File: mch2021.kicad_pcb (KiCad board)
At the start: 2 copper layers, 113.6 x 145.9 mm, 132 parts, among them J1 USB_OTG, J2 AudioJack3, J3 QG-2864KLBEG01, J4 Conn_02x03_Odd_Even, J5 Conn_02x05_Odd_Even, J6 Micro_SD_Card, Q1 Q_DUAL_NPN_NPN_E1B1C2E2B2C1, SW1 SW_SPDT, SW2 RESET_SW, SW3 BL_SWITCH, SW4 SW_SPDT, U1 XT4054K421MR-G, U10 MPR121Q, U11 SY6280AAC, U2 CH340C, U3 SY6280AAC, U4 SY8079, U5 PCM5100, U6 ESP32-WROVER, U7 74LVC1G17, U8 IR1261

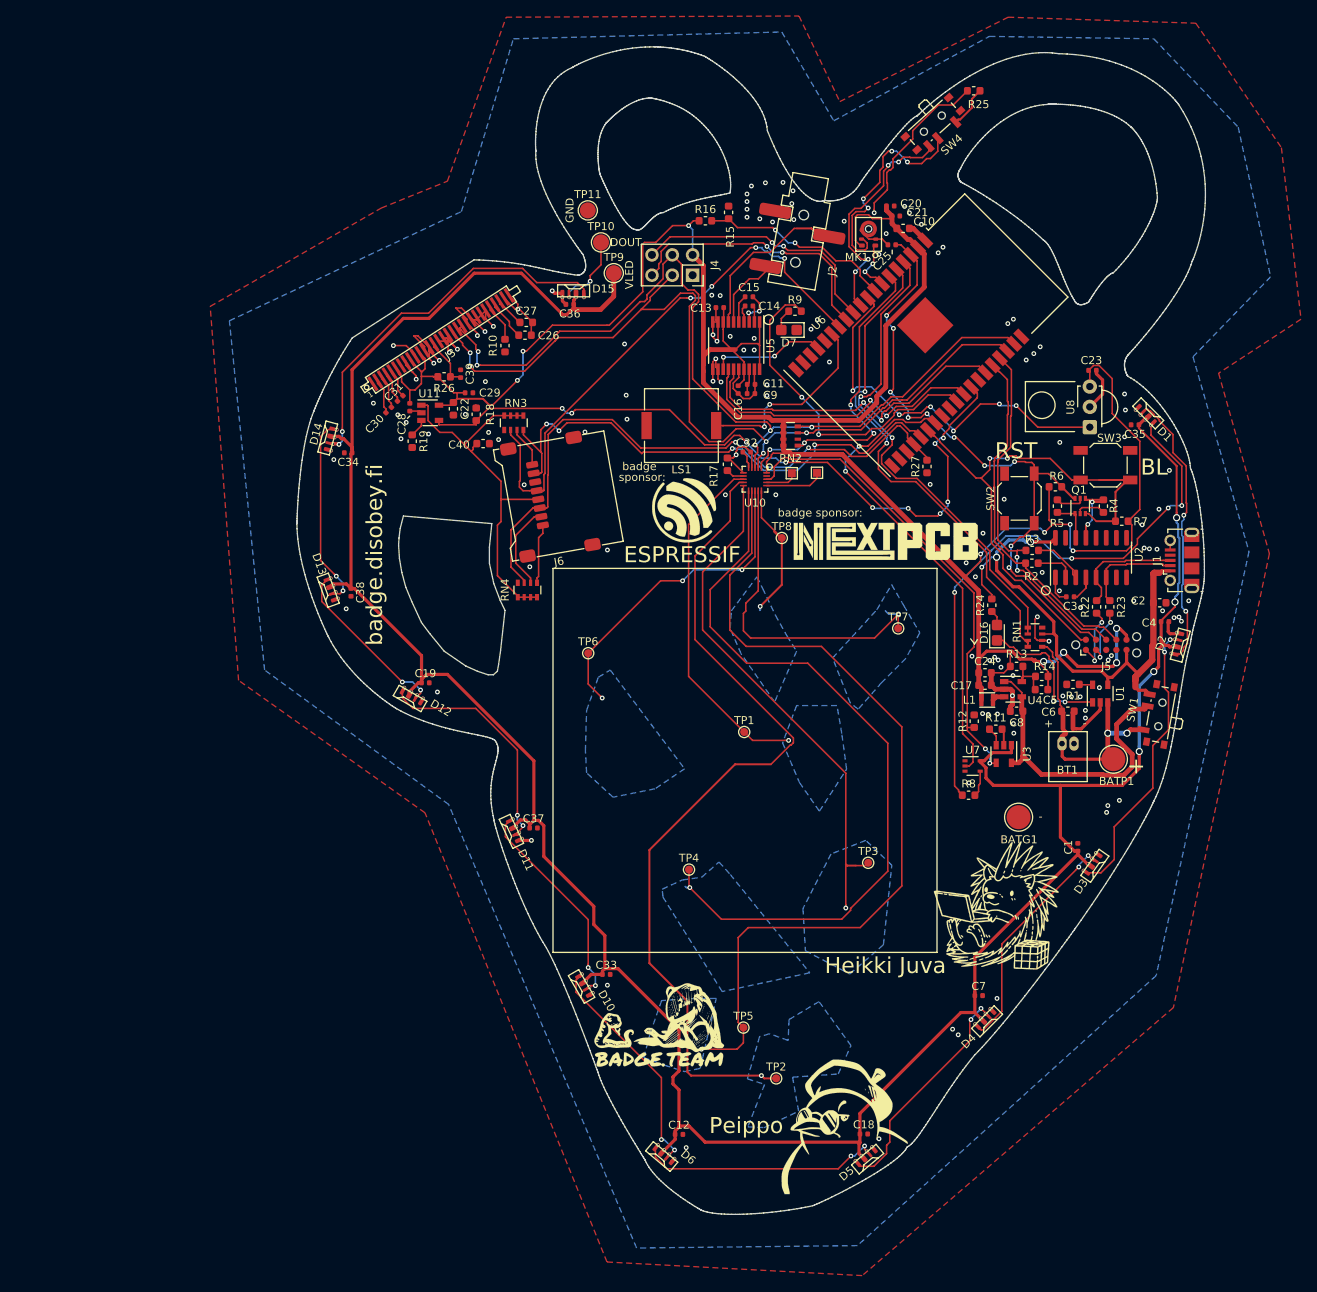
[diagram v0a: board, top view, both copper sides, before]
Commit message: Dump.
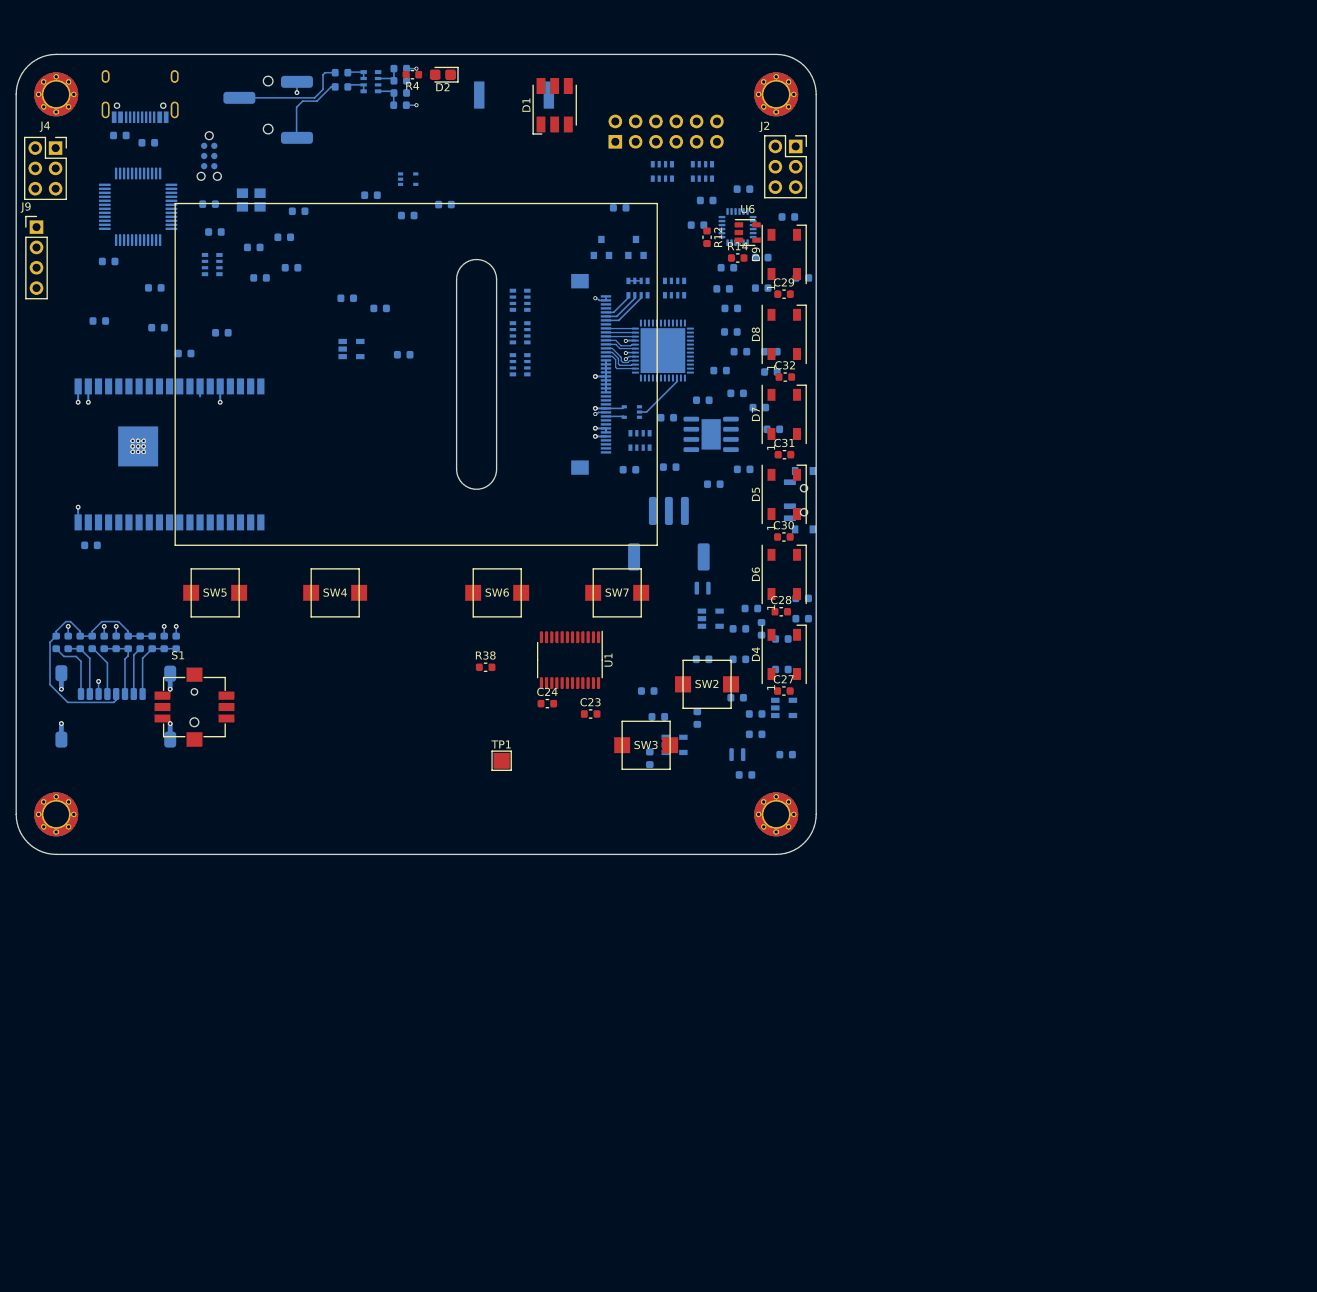
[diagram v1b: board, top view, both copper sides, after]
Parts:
- removed BATG1, BATP1: TestPoint_Flag, TestPoint:TestPoint_Pad_D3.0mm
- removed C22: 100p, Capacitor_SMD:C_0603_1608Metric
- removed C3: 100n, Capacitor_SMD:C_0402_1005Metric
- removed D10, D11, D12, D13, D14, D15: WS2812B, corelib:SK6212SIDE
- removed D16: LED, LED_SMD:LED_0805_2012Metric_Castellated
- removed G***: LOGO, disobey-logo
- removed G***: LOGO, peippo
- removed G***: LOGO, nextpcb
- removed G***: LOGO, badgeteam
- removed G***: LOGO, heikki
- removed G***: LOGO, espressif
- removed G***: LOGO, corp-silk
- removed G***: LOGO, corp-mask
- removed MK1: SPH0641LM4H-1, corelib:Knowles-SPH0641LM4H-1
- removed REF** (x2): TestPoint_Pad_1.0x1.0mm, TestPoint:TestPoint_Pad_1.0x1.0mm
- removed REF**: Battery-48x48mm, corelib:Battery-48x48mm
- removed RN3, RN4: 10k, Resistor_SMD:R_Array_Convex_4x0603
- removed TP10, TP11, TP9: TestPoint, TestPoint:TestPoint_Pad_D2.0mm
- removed TP2, TP3, TP4, TP5, TP6, TP7, TP8: TestPoint_Flag, TestPoint:TestPoint_Pad_D1.0mm
- removed U8: IR1261, OptoDevice:Vishay_MINICAST-3Pin
- added C41: 100n, Capacitor_SMD:C_0603_1608Metric, B.Cu at (90.1, 42.4)
- added C42: 100n, Capacitor_SMD:C_0603_1608Metric, B.Cu at (81.7, 51.6)
- added C43: 20p, Capacitor_SMD:C_0603_1608Metric, B.Cu at (29.7, 24.1)
- added C44: 20p, Capacitor_SMD:C_0603_1608Metric, B.Cu at (33.5, 22.9)
- added C45: 100n, Capacitor_SMD:C_0603_1608Metric, B.Cu at (34.4, 26.7)
- added C46: 100n, Capacitor_SMD:C_0603_1608Metric, B.Cu at (11.6, 25.9)
- added C47: 100n, Capacitor_SMD:C_0603_1608Metric, B.Cu at (30.5, 27.9)
- added D8: WS2812B, LED_SMD:LED_WS2812B_PLCC4_5.0x5.0mm_P3.2mm, F.Cu at (96.0, 35.0)
- added D9: WS2812B, LED_SMD:LED_WS2812B_PLCC4_5.0x5.0mm_P3.2mm, F.Cu at (96.0, 25.0)
- added H1: MountingHole_Pad, corecode:HOLE-M3-COND, F.Cu at (5.00, 5.00)
- added H2: MountingHole_Pad, corecode:HOLE-M3-COND, F.Cu at (95.0, 5.00)
- added H3: MountingHole_Pad, corecode:HOLE-M3-COND, F.Cu at (5.00, 95.0)
- added H4: MountingHole_Pad, corecode:HOLE-M3-COND, F.Cu at (95.0, 95.0)
- added J7: LCD, Connector_FFC-FPC:Hirose_FH12-40S-0.5SH_1x40-1MP_P0.50mm_Horizontal, B.Cu at (71.9, 40.0)
- added J8: PROG, Connector:Tag-Connect_TC2030-IDC-NL_2x03_P1.27mm_Vertical, B.Cu at (24.1, 12.7)
- added J9: GPIO, Connector_PinHeader_2.54mm:PinHeader_1x04_P2.54mm_Vertical, F.Cu at (2.54, 21.6)
- added L2: 2.2u, custom:Inductor_MSC20FC, B.Cu at (90.1, 87.5)
- added Q2: Q_NMOS_GSD, Package_TO_SOT_SMD:SOT-23, B.Cu at (73.2, 24.1)
- added R20: DNP, Resistor_SMD:R_0603_1608Metric, B.Cu at (20.0, 73.5)
- added R21: DNP, Resistor_SMD:R_0603_1608Metric, B.Cu at (12.5, 73.5)
- added R28: 100k, Resistor_SMD:R_0603_1608Metric, B.Cu at (88.0, 39.5)
- added R29: TBD, Resistor_SMD:R_0603_1608Metric, B.Cu at (48.0, 4.83)
- added R30: TBD, Resistor_SMD:R_0603_1608Metric, B.Cu at (48.0, 3.30)
- added R31: 10k, Resistor_SMD:R_0603_1608Metric, B.Cu at (90.5, 37.2)
- added R32: 10k, Resistor_SMD:R_0603_1608Metric, B.Cu at (44.3, 17.6)
- added R33: 10k, Resistor_SMD:R_0603_1608Metric, B.Cu at (48.9, 20.1)
- added R34: 10k, Resistor_SMD:R_0603_1608Metric, B.Cu at (35.3, 19.6)
- added R35: 10k, Resistor_SMD:R_0603_1608Metric, B.Cu at (24.1, 18.7)
- added R36: 10k, Resistor_SMD:R_0603_1608Metric, B.Cu at (17.3, 29.2)
- added R37: 4k7, Resistor_SMD:R_0603_1608Metric, B.Cu at (85.8, 43.2)
- added R38: 4k7, Resistor_SMD:R_0603_1608Metric, F.Cu at (58.7, 76.6)
- added R49: 10k, Resistor_SMD:R_0603_1608Metric, B.Cu at (10.4, 33.3)
- added R50: 10k, Resistor_SMD:R_0603_1608Metric, B.Cu at (25.7, 34.8)
- added R51: 10k, Resistor_SMD:R_0603_1608Metric, B.Cu at (48.4, 37.5)
- added R52: 10k, Resistor_SMD:R_0603_1608Metric, B.Cu at (21.1, 37.4)
- added R53: 10k, Resistor_SMD:R_0603_1608Metric, B.Cu at (9.50, 73.5)
- added R54: 10k, Resistor_SMD:R_0603_1608Metric, B.Cu at (14.0, 73.5)
- added R55: 10k, Resistor_SMD:R_0603_1608Metric, B.Cu at (8.00, 73.5)
- added R56: 10k, Resistor_SMD:R_0603_1608Metric, B.Cu at (5.00, 73.5)
- added R57: 10k, Resistor_SMD:R_0603_1608Metric, B.Cu at (17.0, 73.5)
- added R58: 10k, Resistor_SMD:R_0603_1608Metric, B.Cu at (15.5, 73.5)
- added RN10: 100k, Resistor_SMD:R_Array_Convex_4x0603, B.Cu at (63.0, 30.7)
- added RN11: 100k, Resistor_SMD:R_Array_Convex_4x0603, B.Cu at (63.0, 38.8)
- added RN12: 100k, Resistor_SMD:R_Array_Convex_4x0603, B.Cu at (63.0, 34.8)
- added RN13: 47, Resistor_SMD:R_Array_Convex_4x0603, B.Cu at (85.8, 14.6)
- added RN14: 47, Resistor_SMD:R_Array_Convex_4x0603, B.Cu at (80.8, 14.6)
- added RN7: 47, Resistor_SMD:R_Array_Convex_4x0603, B.Cu at (78.0, 48.3)
- added RN8: 47, Resistor_SMD:R_Array_Convex_4x0603, B.Cu at (77.7, 29.2)
- added RN9: 100k, Resistor_SMD:R_Array_Convex_4x0603, B.Cu at (82.3, 29.2)
- added S1: JS1400BFQ, custom:SW_JS1400BFQ, F.Cu at (22.3, 81.6)
- added SW5: Home, custom:1TS009, F.Cu at (24.9, 67.3)
- added SW6: Start, custom:1TS009, F.Cu at (60.1, 67.3)
- added SW7: Select, custom:1TS009, F.Cu at (75.1, 67.3)
- added U12: LY68L6400, Package_SO:SOIC-8-1EP_3.9x4.9mm_P1.27mm_EP2.41x3.81mm, B.Cu at (86.9, 47.5)
- added U13: 74LVC1G125, Package_TO_SOT_SMD:SOT-353_SC-70-5, B.Cu at (49.0, 15.6)
- added U14: STM32F103C8Tx, Package_QFP:LQFP-48_7x7mm_P0.5mm, B.Cu at (15.2, 19.1)
- added U9: ESP32-WROVER, custom:ESP32-WROVER, B.Cu at (16.0, 50.0)
- added Y1: 16MHz, Crystal:Crystal_SMD_3225-4Pin_3.2x2.5mm, B.Cu at (29.4, 18.2)
- BT1: value Battery_Cell -> LiPo; footprint corelib:S2B-ZR -> Connector_JST:JST_PH_S3B-PH-SM4-TB_1x03-1MP_P2.00mm_Horizontal; moved to B.Cu
- C1, C36, C37: value 1u -> C_Small; footprint Capacitor_SMD:C_0402_1005Metric -> Capacitor_SMD:C_0603_1608Metric; moved to B.Cu
- C10, C6: value 10u -> 22u; moved to B.Cu
- C11, C13: value 100n -> 22u; footprint Capacitor_SMD:C_0402_1005Metric -> Capacitor_SMD:C_0603_1608Metric; moved to B.Cu
- C12, C16: value 1u -> 22u; footprint Capacitor_SMD:C_0402_1005Metric -> Capacitor_SMD:C_0603_1608Metric; moved to B.Cu
- C14, C21, C34, C4: value 1u -> 10u; footprint Capacitor_SMD:C_0402_1005Metric -> Capacitor_SMD:C_0603_1608Metric; moved to B.Cu
- C15, C18, C33, C35, C38, C39, C7: value 1u -> 100n; footprint Capacitor_SMD:C_0402_1005Metric -> Capacitor_SMD:C_0603_1608Metric; moved to B.Cu
- C17, C40: value 22u -> 100n; moved to B.Cu
- C19: value 1u -> 2.2n; footprint Capacitor_SMD:C_0402_1005Metric -> Capacitor_SMD:C_0603_1608Metric; moved to B.Cu
- C2: value 10u -> C_Small; moved to B.Cu
- C20, C25: footprint Capacitor_SMD:C_0402_1005Metric -> Capacitor_SMD:C_0603_1608Metric; moved to B.Cu
- C23: value 1u -> 100n; footprint Capacitor_SMD:C_0402_1005Metric -> Capacitor_SMD:C_0603_1608Metric
- C24: value 22u -> 10u
- C26: value 4.7u -> 10u; moved to B.Cu
- C27: value 2.2u -> 1u
- C28, C29, C30, C31: footprint Capacitor_SMD:C_0402_1005Metric -> Capacitor_SMD:C_0603_1608Metric
- C32: value 100n -> 1u; footprint Capacitor_SMD:C_0402_1005Metric -> Capacitor_SMD:C_0603_1608Metric
- C5: value 22p -> 22u; moved to B.Cu
- C8: value 22u -> 22p; moved to B.Cu
- C9: value 1u -> 22p; footprint Capacitor_SMD:C_0402_1005Metric -> Capacitor_SMD:C_0603_1608Metric; moved to B.Cu
- D1: value WS2812B -> RGB-5050; footprint corelib:SK6212SIDE -> LED_SMD:LED_RGB_5050-6
- D2: value WS2812B -> LED; footprint corelib:SK6212SIDE -> LED_SMD:LED_0805_2012Metric_Castellated
- D3: value WS2812B -> CDBU0130R; footprint corelib:SK6212SIDE -> Diode_SMD:D_0603_1608Metric; moved to B.Cu
- D4, D5, D6: footprint corelib:SK6212SIDE -> LED_SMD:LED_WS2812B_PLCC4_5.0x5.0mm_P3.2mm
- D7: value LED -> WS2812B; footprint LED_SMD:LED_0805_2012Metric_Castellated -> LED_SMD:LED_WS2812B_PLCC4_5.0x5.0mm_P3.2mm
- J1: value USB_OTG -> USB_C_Receptacle_USB2.0; footprint Connector_USB:USB_Micro-B_Molex-105017-0001 -> Connector_USB:USB_C_Receptacle_HRO_TYPE-C-31-M-12; moved to B.Cu
- J2: value AudioJack3 -> SAO; footprint corelib:Boom-audiojack-PJ-320B -> Connector_PinSocket_2.54mm:PinSocket_2x03_P2.54mm_Vertical
- J3: value QG-2864KLBEG01 -> AudioJack3; footprint corelib:hotbar_30x0.7 -> custom:Boom-audiojack-PJ-320B; moved to B.Cu
- J4: value Conn_02x03_Odd_Even -> SAO
- J5: value Conn_02x05_Odd_Even -> Micro SD card; footprint Connector:Tag-Connect_TC2050-IDC-NL_2x05_P1.27mm_Vertical -> custom:MicroSD-SOFNG-TF-002-H18; moved to B.Cu
- J6: value Micro_SD_Card -> PMOD; footprint corelib:MicroSD-SOFNG-TF-002-H18 -> Connector_PinSocket_2.54mm:PinSocket_2x06_P2.54mm_Horizontal; moved to B.Cu
- L1: footprint corelib:Inductor_MSC20FC -> custom:Inductor_MSC20FC; moved to B.Cu
- LS1, R13, R6, R7: moved to B.Cu
- Q1: value Q_DUAL_NPN_NPN_E1B1C2E2B2C1 -> Q_NMOS_GSD; footprint Package_TO_SOT_SMD:SOT-363_SC-70-6 -> Package_TO_SOT_SMD:SOT-23; moved to B.Cu
- R1: value 2k -> 5k1; moved to B.Cu
- R10: value 910k -> 2k; moved to B.Cu
- R11: value 3.4k -> 10k; moved to B.Cu
- R14: value 45.3k -> 3.4k
- R15: value R -> 4k7; moved to B.Cu
- R16: value 10k -> 4k7; moved to B.Cu
- R17: value 75k -> 4k7; moved to B.Cu
- R18, R19: value 10k -> 45.3k; moved to B.Cu
- R2: value 100R -> 5k1; moved to B.Cu
- R22: value 0 -> 45.3k; moved to B.Cu
- R23: value 0 -> 47; moved to B.Cu
- R24: value 2K -> 47; moved to B.Cu
- R25: value 10k -> 100k; moved to B.Cu
- R26: value 10k -> 100; moved to B.Cu
- R27: value 45.3k -> 100k; moved to B.Cu
- R3: value 100R -> 47; moved to B.Cu
- R4: value 10k -> 100
- R5: value 10k -> 2k; moved to B.Cu
- R8: value 1k -> 45.3k; moved to B.Cu
- R9: value 100R -> 10k; moved to B.Cu
- RN1: value 100k -> TBD; moved to B.Cu
- RN2: value 4.7k -> 100k; moved to B.Cu
- SW1: value SW_SPDT -> Power switch; moved to B.Cu
- SW2: value RESET_SW -> Accept; footprint Button_Switch_SMD:SW_SPST_SKQG_WithStem -> custom:1TS009
- SW3: value BL_SWITCH -> Back; footprint Button_Switch_SMD:SW_SPST_SKQG_WithStem -> custom:1TS009
- SW4: value SW_SPDT -> Menu; footprint Button_Switch_SMD:SW_SPDT_PCM12 -> custom:1TS009
- TP1: value TestPoint_Flag -> IOEXP; footprint TestPoint:TestPoint_Pad_D1.0mm -> TestPoint:TestPoint_Pad_2.0x2.0mm
- U1: value XT4054K421MR-G -> PCA9555PW; footprint Package_TO_SOT_SMD:SOT-23-5 -> Package_SO:TSSOP-24_4.4x7.8mm_P0.65mm
- U10: value MPR121Q -> 74LVC1G125; footprint Package_DFN_QFN:QFN-20-1EP_3x3mm_P0.4mm_EP1.65x1.65mm -> Package_TO_SOT_SMD:SOT-353_SC-70-5; moved to B.Cu
- U11: value SY6280AAC -> ICE40UP5K-SG48ITR; footprint Package_TO_SOT_SMD:SOT-23-5 -> Package_DFN_QFN:QFN-48-1EP_7x7mm_P0.5mm_EP5.6x5.6mm; moved to B.Cu
- U2: value CH340C -> SY8079AAC; footprint Package_SO:SOIC-16_3.9x9.9mm_P1.27mm -> Package_TO_SOT_SMD:SOT-23-5; moved to B.Cu
- U3: value SY6280AAC -> SY8079AAC; moved to B.Cu
- U4: value SY8079 -> XT4054K421MR-G; moved to B.Cu
- U5: value PCM5100 -> SY6280AAC; footprint Package_SO:TSSOP-20_4.4x6.5mm_P0.65mm -> Package_TO_SOT_SMD:SOT-23-5; moved to B.Cu
- U6: value ESP32-WROVER -> SY6280AAC; footprint corelib:ESP32-WROVER -> Package_TO_SOT_SMD:SOT-23-5
- U7: value 74LVC1G17 -> MPU-6050; footprint Package_TO_SOT_SMD:SOT-353_SC-70-5 -> Sensor_Motion:InvenSense_QFN-24_4x4mm_P0.5mm; moved to B.Cu
- moved J1 143.1 mm to (15.5, 3.81), turned to 0 degrees
- moved R1 137.5 mm to (13.0, 10.1), turned to 0 degrees
- moved C1 132.3 mm to (40.7, 4.06), turned to 180 degrees
- moved R22 124.1 mm to (11.0, 73.5)
- moved J5 123.9 mm to (12.5, 80.0)
- moved R2 122.3 mm to (16.5, 11.0)
- moved C2 121.9 mm to (40.7, 2.29)
- moved D2 117.0 mm to (53.3, 2.54), turned to 180 degrees
- moved C18 110.3 mm to (93.2, 25.4)
- moved RN1 108.2 mm to (44.3, 3.41), turned to 0 degrees
- moved D3 101.8 mm to (75.4, 19.2), turned to 0 degrees
- moved R4 101.8 mm to (49.5, 2.54), turned to 180 degrees
- moved R11 97.3 mm to (41.4, 30.5)
- moved C37 96.4 mm to (48.0, 1.78), turned to 180 degrees
- moved SW4 95.0 mm to (39.9, 67.3), turned to 0 degrees
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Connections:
- BT1 pad 1: /BAT -> +3V3
- C1 pad 1: VCC -> Net-(C1-Pad1)
- C1 pad 2: GND -> Net-(C1-Pad2)
- C10 pad 1: /3V3 -> +3V3
- C11 pad 1: Net-(C11-Pad1) -> +1V2
- C12 pad 1: VCC -> +3V3
- C13 pad 1: /3V3 -> +1V2
- C14 pad 1: Net-(C14-Pad1) -> +3V3
- C14 pad 2: Net-(C14-Pad2) -> GND
- C15 pad 1: Net-(C15-Pad1) -> +3V3
- C16 pad 1: /3V3 -> PWR_SDCARD
- C17 pad 1: /3V3 -> +3V3
- C18 pad 1: VCC -> GND
- C18 pad 2: GND -> Net-(C18-Pad2)
- C19 pad 1: VCC -> GND
- C19 pad 2: GND -> Net-(C19-Pad2)
- C2 pad 1: /VUSB -> Net-(C2-Pad1)
- C2 pad 2: GND -> Net-(C2-Pad2)
- C20 pad 1: /3V3 -> +3V3
- C21 pad 1: /3V3 -> +3V3
- C23 pad 1: GND -> +3V3
- C23 pad 2: /3V3 -> GND
- C24 pad 1: /3V3 -> +3V3
- C25 pad 1: /RESET -> +3V3
- C26 pad 1: Net-(C26-Pad1) -> +3V3
- C27 pad 1: Net-(C27-Pad1) -> PWR_LED
- C28 pad 1: /3V3 -> PWR_LED
- C29 pad 1: /3V3 -> PWR_LED
- C30 pad 1: Net-(C30-Pad1) -> PWR_LED
- C30 pad 2: Net-(C30-Pad2) -> GND
- C31 pad 1: Net-(C31-Pad1) -> PWR_LED
- C31 pad 2: Net-(C31-Pad2) -> GND
- C32 pad 1: Net-(C32-Pad1) -> PWR_LED
- C33 pad 1: VCC -> +1V2
- C34 pad 1: VCC -> Net-(C34-Pad1)
- C35 pad 1: VCC -> Net-(C34-Pad1)
- C36 pad 1: VCC -> GND
- C36 pad 2: GND -> /FPGA/AUDO_L
- C37 pad 1: VCC -> GND
- C37 pad 2: GND -> /FPGA/AUDO_R
- C38 pad 1: VCC -> +3V3
- C39 pad 1: GND -> +3V3
- C39 pad 2: Net-(C39-Pad2) -> GND
- C4 pad 1: VCC -> GND
- C4 pad 2: GND -> VUSB
- C40 pad 1: /GATEDPOWER -> +3V3
- C5 pad 1: /3V3 -> VIN
- C5 pad 2: Net-(C5-Pad2) -> GND
- C6 pad 1: /BAT -> VIN
- C7 pad 1: VCC -> GND
- C7 pad 2: GND -> VUSB
- C8 pad 1: /BATSW -> +3V3
- C8 pad 2: GND -> /POWER/FB33
- C9 pad 1: Net-(C11-Pad1) -> +1V2
- C9 pad 2: GND -> /POWER/FB12
- D1 pad 1: VCC -> /FPGA/RGB2
- D1 pad 2: Net-(D1-Pad2) -> /FPGA/RGB0
- D1 pad 3: GND -> /FPGA/RGB1
- D1 pad 4: /LED_DIN -> +3V3
- D2 pad 1: VCC -> GND
- D3 pad 1: VCC -> +2V5
- D3 pad 2: Net-(D3-Pad2) -> +3V3
- D4 pad 1: VCC -> PWR_LED
- D4 pad 4: Net-(D3-Pad2) -> /LED/DATA_IN
- D5 pad 1: VCC -> PWR_LED
- D6 pad 1: VCC -> PWR_LED
- D6 pad 2: Net-(D10-Pad4) -> Net-(D6-Pad2)
- D7 pad 1: GND -> PWR_LED
- J4 pad 2: /3V3 -> +3V3
- J4 pad 3: /SCL -> /ACCELEROMETER/I2C_SCL
- J4 pad 4: /SDA -> /ACCELEROMETER/I2C_SDA
- J4 pad 5: Net-(J4-Pad5) -> /STM32/SAO_IO0
- J4 pad 6: Net-(J4-Pad6) -> /STM32/SAO_IO1
- J5 pad 1: Net-(J5-Pad1) -> SD_D2
- J5 pad 2: Net-(J5-Pad2) -> /ESP32/SD_D3
- J5 pad 3: GND -> SD_CMD
- J5 pad 4: GND -> PWR_SDCARD
- J5 pad 5: /VUSB -> /ESP32/SD_CLK
- J5 pad 6: /3V3 -> GND
- J5 pad 7: /ESPRX -> SD_D0
- J5 pad 8: /ESPTX -> /ESP32/SD_D1
- J5 pad 9: /RESET -> GND
- J6 pad 1: Net-(J6-Pad1) -> +3V3
- J6 pad 2: Net-(J6-Pad2) -> +3V3
- J6 pad 3: /SD_CMD -> GND
- J6 pad 4: /GATEDPOWER -> GND
- J6 pad 5: /SD_CLK -> /FPGA/PMOD_8
- J6 pad 6: GND -> /FPGA/PMOD_4
- J6 pad 7: /SD_D0 -> /FPGA/PMOD_7
- J6 pad 8: Net-(J6-Pad8) -> /FPGA/PMOD_3
- J6 pad 9: GND -> /FPGA/PMOD_6
- L1 pad 1: /3V3 -> +3V3
- L1 pad 2: Net-(L1-Pad2) -> /POWER/SW33
- LS1 pad 1: /BUZZER -> GND
- LS1 pad 2: GND -> SPK
- Q1 pad 2: Net-(Q1-Pad2) -> GND
- Q1 pad 3: /BL -> Net-(Q1-Pad3)
- R1 pad 1: Net-(R1-Pad1) -> GND
- R1 pad 2: GND -> /CC1
- R10 pad 1: Net-(J3-Pad26) -> /POWER/CHARGING
- R10 pad 2: GND -> +3V3
- R11 pad 1: Net-(R11-Pad1) -> GND
- R11 pad 2: GND -> /ESP32/PWR_SDCARD_ENABLE
- R12 pad 1: /LEDON -> GND
- R12 pad 2: GND -> /POWER/PWR_LED_ENABLE
- R13 pad 1: Net-(C5-Pad2) -> GND
- R13 pad 2: GND -> Net-(R13-Pad2)
- R14 pad 1: /3V3 -> Net-(R14-Pad1)
- R14 pad 2: Net-(C5-Pad2) -> GND
- R15 pad 1: Net-(R15-Pad1) -> +3V3
- R15 pad 2: GND -> /ACCELEROMETER/AUX_SDA
- R16 pad 1: /3V3 -> +3V3
- R16 pad 2: Net-(R15-Pad1) -> /ACCELEROMETER/AUX_SCL
- R17 pad 1: Net-(R17-Pad1) -> +3V3
- R17 pad 2: GND -> /ACCELEROMETER/IRQ
- R18 pad 1: Net-(R18-Pad1) -> SD_D0
- R19 pad 1: Net-(R19-Pad1) -> +3V3
- R19 pad 2: GND -> SD_D2
- R2 pad 1: /ESPRX -> GND
- R2 pad 2: Net-(R2-Pad2) -> /CC2
- R22 pad 1: Net-(J5-Pad1) -> SD_CMD
- R22 pad 2: /D_P -> GND
- R23 pad 1: /D_N -> /LCD/LCD_RS_SCK
- R23 pad 2: Net-(J5-Pad2) -> /FPGA/LCD_RS
- R24 pad 1: Net-(D16-Pad2) -> /LCD/LCD_IM0
- R24 pad 2: /VUSB -> /STM32/LCD_MODE
- R25 pad 1: GND -> /FPGA/SPI_CS
- R25 pad 2: Net-(R25-Pad2) -> GND
- R26 pad 1: Net-(C39-Pad2) -> +1V2
- R26 pad 2: /3V3 -> Net-(C34-Pad1)
- R27 pad 1: GND -> /BUTTONS/FPGA_RESET
- R27 pad 2: /SD_CMD -> GND
- R3 pad 1: /ESPTX -> Net-(J2-Pad6)
- R3 pad 2: Net-(R3-Pad2) -> /LED/DATA_OUT
- R4 pad 1: Net-(Q1-Pad2) -> Net-(D2-Pad2)
- R4 pad 2: Net-(Q1-Pad4) -> /ESP32/IR_TX
- R5 pad 1: Net-(Q1-Pad5) -> Net-(R5-Pad1)
- R5 pad 2: Net-(Q1-Pad1) -> GND
- R6 pad 1: /RESET -> /POWER/FB33
- R6 pad 2: /3V3 -> GND
- R7 pad 1: /BL -> /POWER/FB12
- R7 pad 2: /3V3 -> GND
- R8 pad 1: /LED_DIN -> +3V3
- R8 pad 2: Net-(R8-Pad2) -> /POWER/FB33
- R9 pad 1: Net-(D7-Pad2) -> +1V2
- R9 pad 2: /IR_SEND -> /POWER/FB12
- RN1 pad 1: /BAT -> Net-(C1-Pad1)
- RN1 pad 2: GND -> Net-(C1-Pad1)
- RN1 pad 3: /VUSB -> Net-(C2-Pad2)
- RN1 pad 4: GND -> Net-(C2-Pad2)
- RN1 pad 5: /USB_SENSE -> ESP32_AUDIO_R
- RN1 pad 6: /USB_SENSE -> /FPGA/AUDO_R
- RN1 pad 7: /BATSENSE -> ESP32_AUDIO_L
- RN1 pad 8: /BATSENSE -> /FPGA/AUDO_L
- RN2 pad 1: /TOUCHRDY -> +3V3
- RN2 pad 2: Net-(RN2-Pad2) -> GND
- RN2 pad 3: /SCL -> VUSB
- RN2 pad 4: /SDA -> GND
- RN2 pad 5: /3V3 -> /POWER/SENSE_VUSB
- RN2 pad 6: /3V3 -> /POWER/SENSE_VUSB
- RN2 pad 7: /3V3 -> /POWER/SENSE_VBAT
- RN2 pad 8: /3V3 -> /POWER/SENSE_VBAT
- SW1 pad 1: /BAT -> +3V3
- SW1 pad 2: /BATSW -> VIN
- SW1 pad 3: /VUSB -> VUSB
- SW2 pad 1: GND -> Net-(SW2-Pad1)
- SW2 pad 2: /RESET -> GND
- SW3 pad 1: GND -> Net-(SW3-Pad1)
- SW3 pad 2: /BL -> GND
- SW4 pad 1: Net-(R25-Pad2) -> Net-(SW4-Pad1)
- SW4 pad 2: Net-(MK1-Pad4) -> GND
- TP1 pad 1: /T-UP -> Net-(TP1-Pad1)
- U1 pad 1: Net-(D16-Pad1) -> /BUTTONS/IRQ
- U1 pad 3: /BAT -> GND
- U1 pad 4: /VUSB -> Net-(S1-Pad1)
- U1 pad 5: Net-(R1-Pad1) -> Net-(S1-Pad2)
- U10 pad 1: /TOUCHRDY -> /LCD/LCD_RS_SCK_SWITCH
- U10 pad 2: /SCL -> /ESP32/SPI_CLK
- U10 pad 3: /SDA -> GND
- U10 pad 4: GND -> /LCD/LCD_RS_SCK
- U10 pad 5: Net-(C32-Pad1) -> +3V3
- U11 pad 1: /GATEDPOWER -> +3V3
- U11 pad 2: GND -> Net-(RN14-Pad3)
- U11 pad 3: Net-(R19-Pad1) -> Net-(RN14-Pad1)
- U11 pad 4: Net-(R18-Pad1) -> Net-(RN14-Pad2)
- U11 pad 5: /3V3 -> +1V2
- U2 pad 1: GND -> VIN
- U2 pad 2: Net-(R2-Pad2) -> GND
- U2 pad 3: Net-(R3-Pad2) -> /POWER/SW33
- U2 pad 4: Net-(C3-Pad1) -> VIN
- U2 pad 5: /D_P -> /POWER/FB33
- U3 pad 1: VCC -> VIN
- U3 pad 3: Net-(R11-Pad1) -> /POWER/SW12
- U3 pad 4: /LEDON -> VIN
- U3 pad 5: /BATSW -> /POWER/FB12
- U4 pad 1: /BATSW -> /POWER/CHARGING
- U4 pad 3: Net-(L1-Pad2) -> +3V3
- U4 pad 4: /BATSW -> VUSB
- U4 pad 5: Net-(C5-Pad2) -> Net-(R5-Pad1)
- U5 pad 1: /3V3 -> PWR_SDCARD
- U5 pad 2: Net-(C14-Pad1) -> GND
- U5 pad 3: GND -> Net-(R13-Pad2)
- U5 pad 4: Net-(C14-Pad2) -> /ESP32/PWR_SDCARD_ENABLE
- U5 pad 5: Net-(C15-Pad1) -> +3V3
- U6 pad 1: GND -> PWR_LED
- U6 pad 2: /3V3 -> GND
- U6 pad 3: /RESET -> Net-(R14-Pad1)
- U6 pad 4: /USB_SENSE -> /POWER/PWR_LED_ENABLE
- U6 pad 5: /BATSENSE -> +3V3
- U7 pad 1: (no net) -> GND
- U7 pad 2: Net-(U6-Pad26) -> (no net)
- U7 pad 3: GND -> (no net)
- U7 pad 4: Net-(R8-Pad2) -> (no net)
- U7 pad 5: VCC -> (no net)
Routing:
- net VCC: track 351.3 -> 0.00 mm, vias 4 -> 0
- net /3V3: track 323.1 -> 0.00 mm, vias 11 -> 0
- net GND: track 158.6 -> 29.6 mm, vias 134 -> 25
- net /SCL: track 112.1 -> 0.00 mm, vias 5 -> 0
- net /SDA: track 111.7 -> 0.00 mm, vias 5 -> 0
- net /T-A: track 107.1 -> 0.00 mm, vias 1 -> 0
- net /T-DOWN: track 105.2 -> 0.00 mm, vias 1 -> 0
- net /T-RIGHT: track 95.2 -> 0.00 mm, vias 1 -> 0
- net Net-(R18-Pad1): track 91.1 -> 0.00 mm, vias 10 -> 0
- net /RESET: track 80.9 -> 0.00 mm, vias 10 -> 0
- net /SD_CMD: track 78.7 -> 0.00 mm, vias 2 -> 0
- net /LED_DIN: track 74.4 -> 0.00 mm, vias 4 -> 0
- net /SD_CLK: track 69.7 -> 0.00 mm, vias 4 -> 0
- net /VUSB: track 67.8 -> 0.00 mm, vias 3 -> 0
- net /BL: track 67.8 -> 0.00 mm, vias 2 -> 0
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- added copper zone on In2.Cu, net +3V3
- added copper zone on In1.Cu, net GND
- removed copper zone on B.Cu, net /T-A
- removed copper zone on B.Cu, net /T-B
- removed copper zone on B.Cu, net /T-DOWN
- removed copper zone on B.Cu, net /T-LEFT
- removed copper zone on B.Cu, net /T-RIGHT
- removed copper zone on B.Cu, net /T-SELECT
- removed copper zone on B.Cu, net /T-START
- removed copper zone on B.Cu, net /T-UP
- removed copper zone on B.Cu, net GND
- removed copper zone on F.Cu, net GND
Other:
- board size 113.6 x 145.9 mm -> 100 x 100 mm
- copper layers 2 -> 4
- board text removed: "+"
- board text removed: "-"
- board text removed: "A"
- board text removed: "AUDIO"
- board text removed: "B"
- board text removed: "BL"
- board text removed: "DOUT"
- board text removed: "DOWN"
- board text removed: "ESPRESSIF"
- board text removed: "GND"
- board text removed: "Heikki Juva"
- board text removed: "Jaga"
- board text removed: "Kliment"
- board text removed: "LEFT"
- board text removed: "MIC"
- board text removed: "OFF"
- board text removed: "ON"
- board text removed: "Peippo"
- board text removed: "Purkkaviritys"
- board text removed: "RIGHT"
- board text removed: "RST"
- board text removed: "Renze"
- board text removed: "SAC1.69b"
- board text removed: "SELECT"
- board text removed: "START"
- board text removed: "UP"
- board text removed: "USB"
- board text removed: "VLED"
- board text removed: "badge"
- board text removed: "badge sponsor:"
- board text removed: "badge.disobey.fi"
- board text removed: "credits:"
- board text removed: "sponsor:"
